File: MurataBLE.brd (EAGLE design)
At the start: 50 x 31 mm, 33 parts, among them IC1 IC_LDO_XX1117, IC3 74LVC1G04DCK, Q2 12MHz, SW1 SW_TACTSW_2PP8073, SW2 SW_TACTSW_2PP8073, SW3 SW_TACTSW_2PP8073, U1 IC_BLE_LBCA2HNZYZ-711, X1 TSW-112-02-S-S

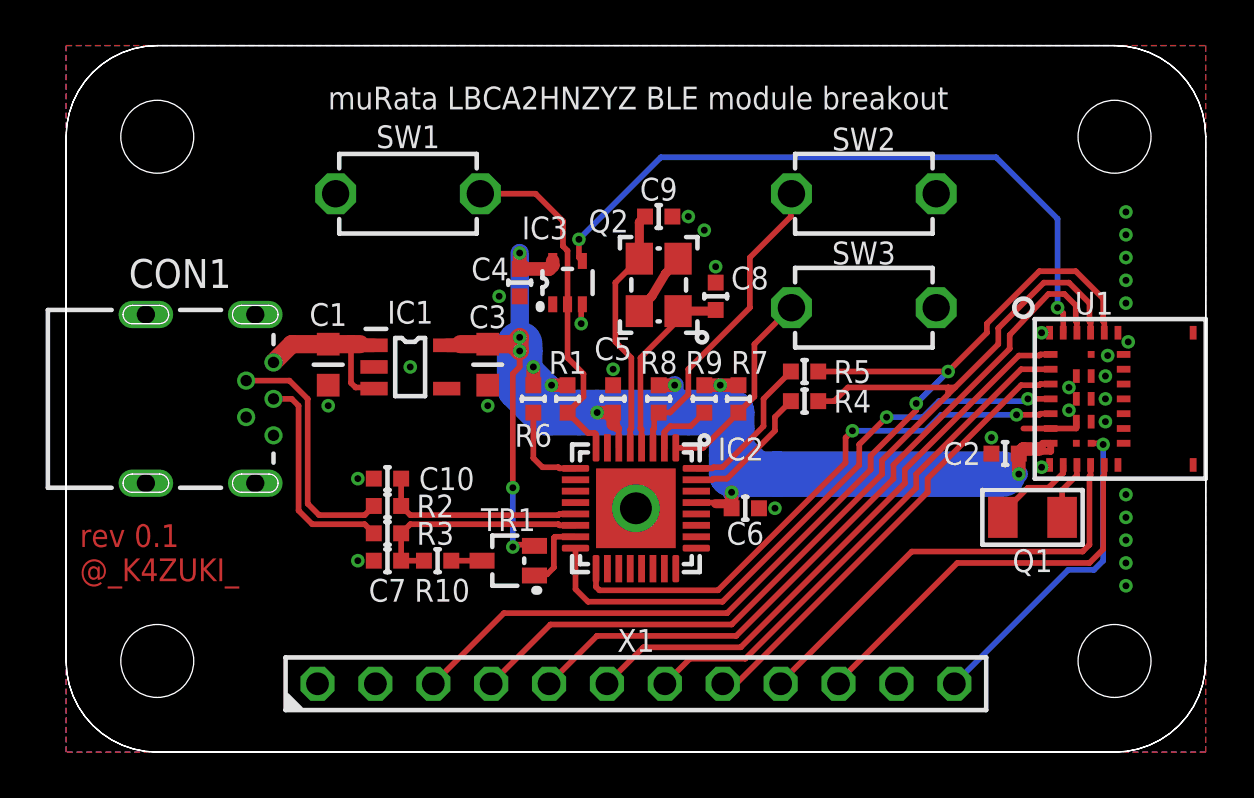
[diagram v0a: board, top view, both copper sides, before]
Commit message: [ FIX ] library update
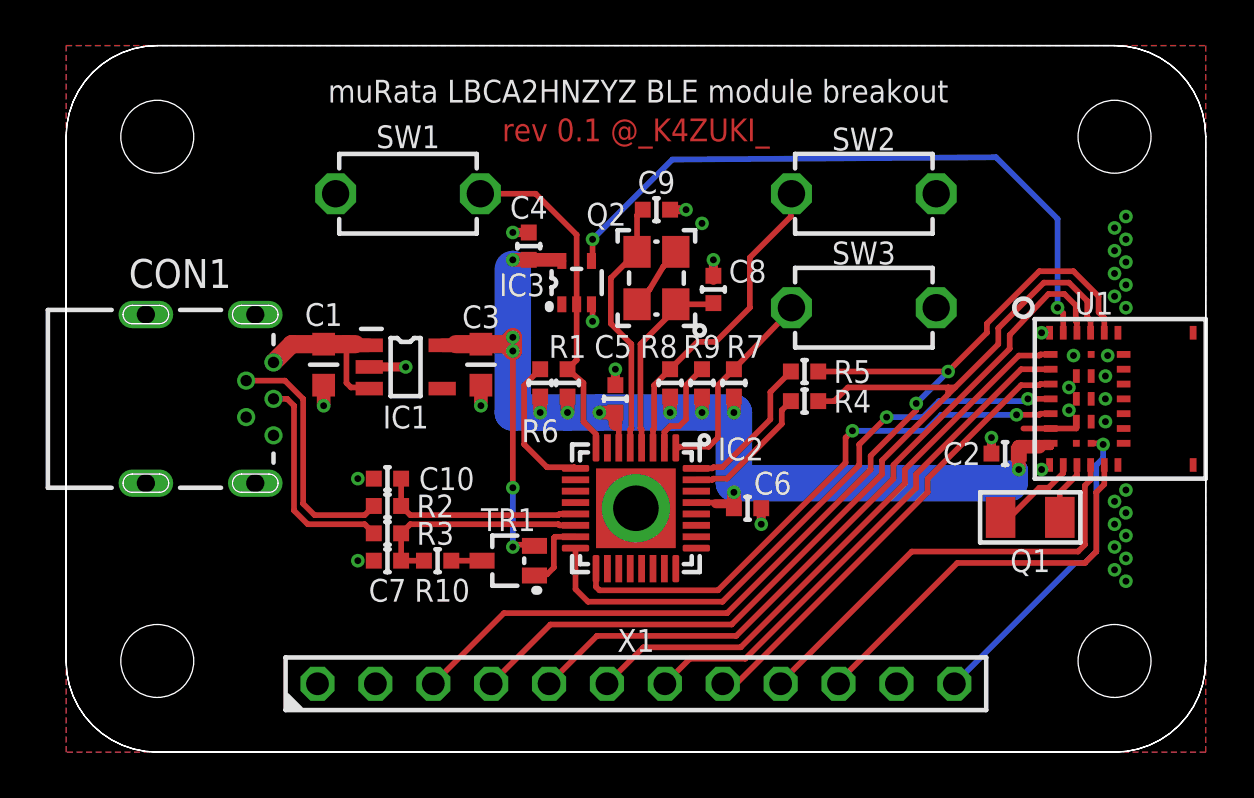
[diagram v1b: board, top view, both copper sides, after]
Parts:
- moved C4 1.65 mm to (20.3, 22.2), turned to 90 degrees
- moved R8 0.86 mm to (26.5, 16.2), turned to 90 degrees
- moved R6 0.76 mm to (20.8, 16.2), turned to 90 degrees
- moved R7 0.73 mm to (29.3, 16.2), turned to 90 degrees
- moved R9 0.71 mm to (27.9, 16.2), turned to 90 degrees
- moved R1 0.70 mm to (22.0, 16.2), turned to 90 degrees
- moved IC3 0.40 mm to (22.4, 20.6)
- moved C8 0.32 mm to (28.4, 20.3)
- moved C9 0.32 mm to (25.9, 23.8)
- moved Q2 0.32 mm to (25.9, 20.8)
- moved C3 0.30 mm to (18.2, 17.0)
- moved C1 0.20 mm to (11.3, 17.0)
- moved IC1 0.20 mm to (14.9, 16.9)
- moved C5 0.10 mm to (24.1, 15.5)
- moved Q1 0.10 mm to (42.3, 10.3)
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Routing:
- net 3.3V: track 72.1 -> 60.9 mm, vias 12 -> 13
- net GND: track 6.45 -> 14.0 mm, vias 33 -> 41
- net N$4: track 4.04 -> 6.27 mm
- net N$5: track 2.80 -> 4.37 mm
- net RESET: track 29.7 -> 29.0 mm
